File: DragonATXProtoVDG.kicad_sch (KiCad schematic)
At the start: 45 parts, among them IC1 74LS273, IC2 MC6847, IC3 MC14053, J3 JTAG, U1 AD724JR, U2 LMH1251, U3 ATF1504ASL-xAx44, Y2 4.433618MHz

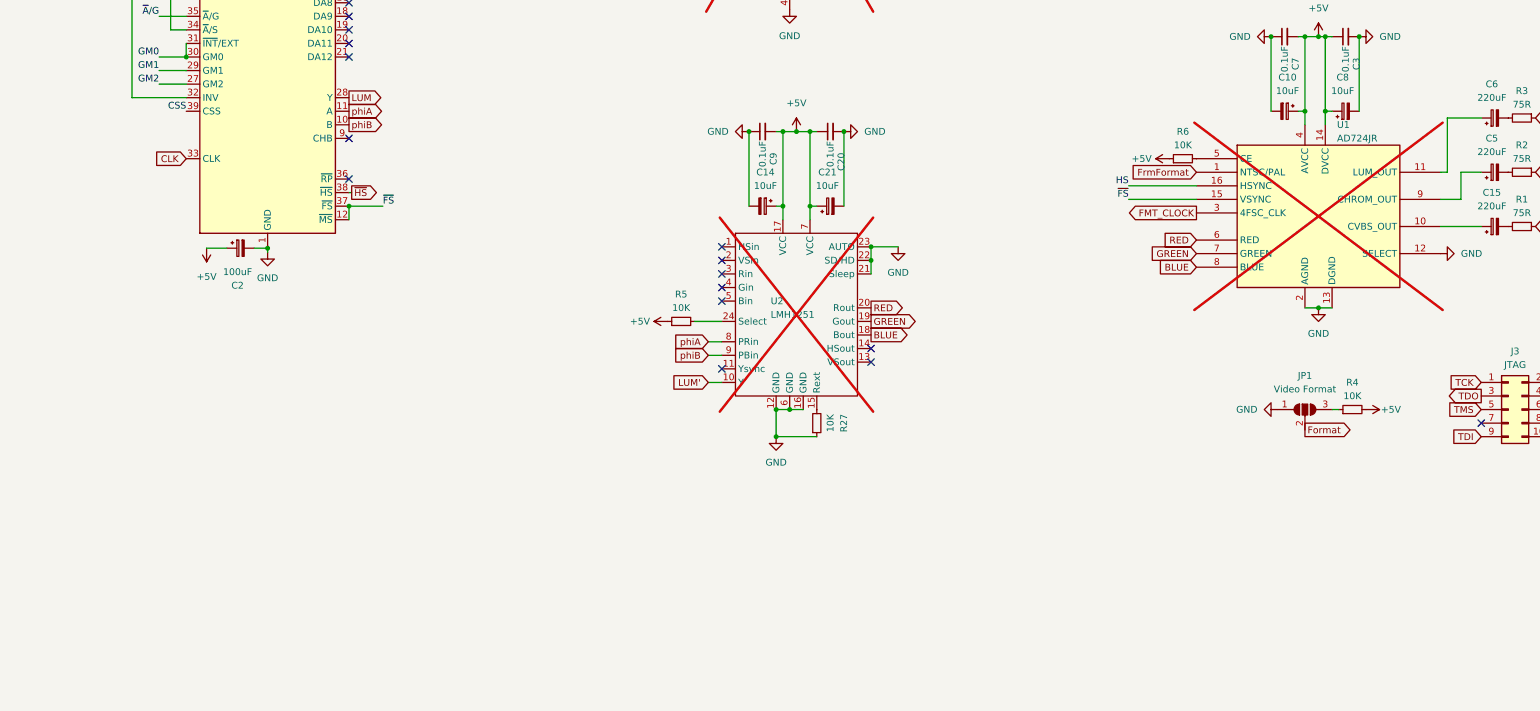
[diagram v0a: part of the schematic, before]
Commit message: condition rgb
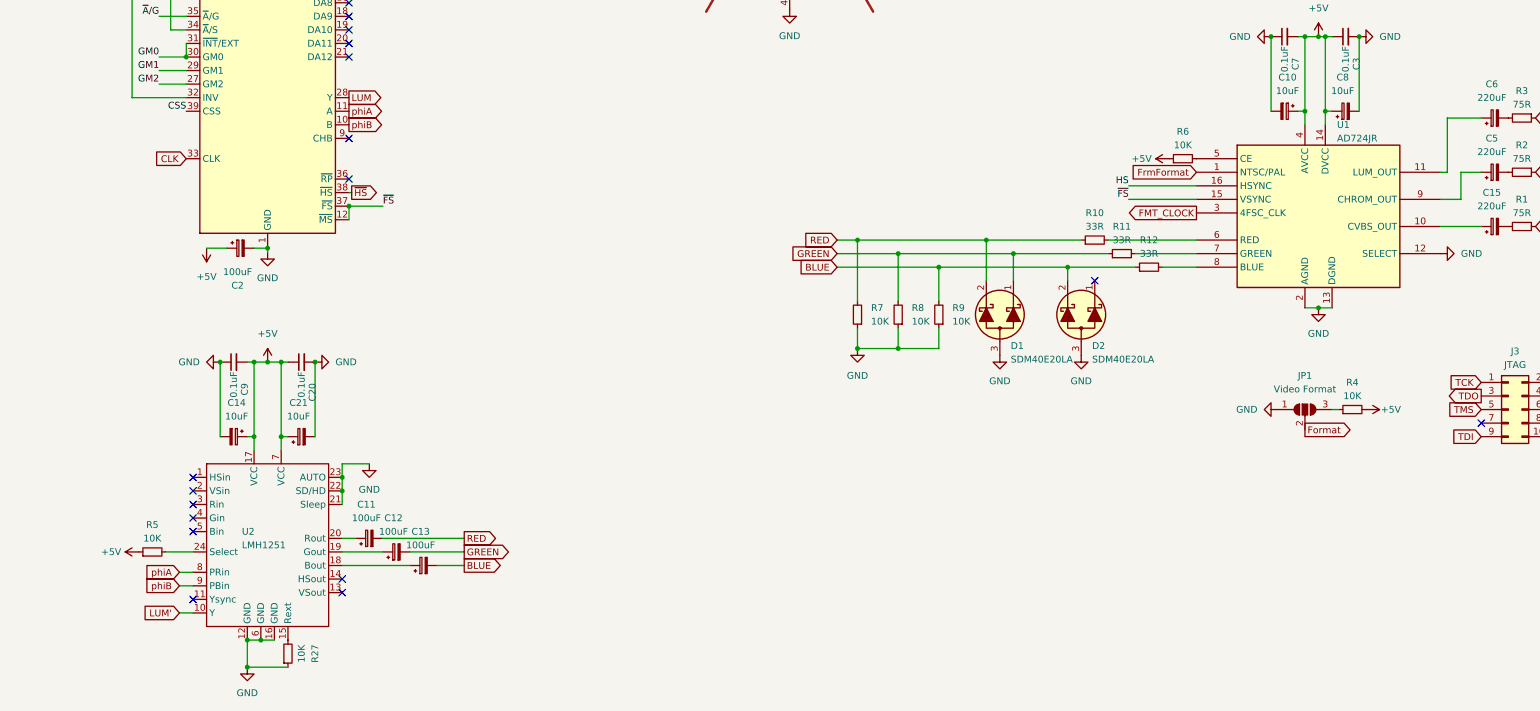
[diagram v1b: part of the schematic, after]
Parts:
- added C11, C12, C13: 100uF, Capacitor_Tantalum_SMD:CP_EIA-2012-12_Kemet-R, symbol Device:C_Polarized_Small
- added D1, D2: SDM40E20LA, PCM_Package_TO_SOT_SMD_AKL:SOT-23, symbol PCM_Diode_Schottky_AKL:SDM40E20LA
- added R10, R11, R12: 33R, Resistor_SMD:R_0805_2012Metric_Pad1.20x1.40mm_HandSolder, symbol Device:R_Small
- added R7, R8, R9: 10K, Resistor_SMD:R_0805_2012Metric_Pad1.20x1.40mm_HandSolder, symbol Device:R_Small
- U1, U2: now fitted
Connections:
- net BLUE: now also C13.2, D2.2 (K2), R12.1, R9.2; no longer U1.8 (BLUE), U2.18 (Bout)
- net GND: now also D1.3 (A), D2.3 (A), R7.1, R8.1, R9.1
- net GREEN: now also C12.2, D1.1 (K1), R11.1, R8.2; no longer U1.7 (GREEN), U2.19 (Gout)
- net RED: now also C11.2, D1.2 (K2), R10.1, R7.2; no longer U1.6 (RED), U2.20 (Rout)
- new net: R12.2, U1.8 (BLUE)
- new net: C12.1, U2.19 (Gout)
- new net: C11.1, U2.20 (Rout)
- new net: R10.2, U1.6 (RED)
- new net: R11.2, U1.7 (GREEN)
- new net: C13.1, U2.18 (Bout)
- no-connect marks 64 -> 65
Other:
- moved on the sheet: C14, C20, C21, C9, R27, R5
